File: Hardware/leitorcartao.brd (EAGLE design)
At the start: 34.5 x 68 mm, 168 parts, among them IC1 TL084, IC2 TL084, Q1 BSH103, Q2 BC847ASMD, Q3 BC857ALT1SMD, Q4 BC847ALT1SMD, Q5 BC847ALT1SMD, Q6 BC847ALT1SMD, Q7 BC847ALT1SMD, Q8 BC847ALT1SMD, U1 SAMD20E14A-AUT, U3 TLV1117-50CDCYR, U4 MFRC52202HN1, U5 LP2985-33DBVR, X1 ANTENA 125kHz, X2 MIFARE ANTENA

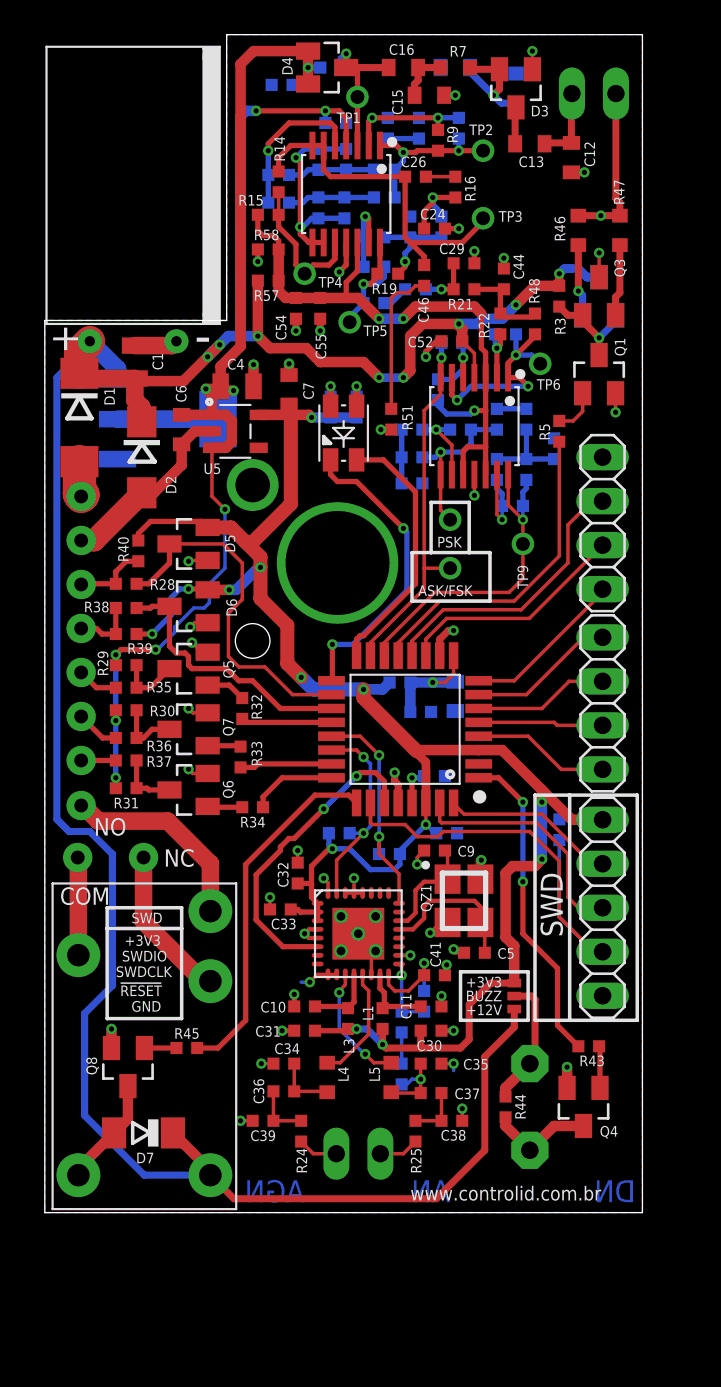
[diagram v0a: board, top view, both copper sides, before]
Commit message: Nova versão do leitor. Aguardando revisão.
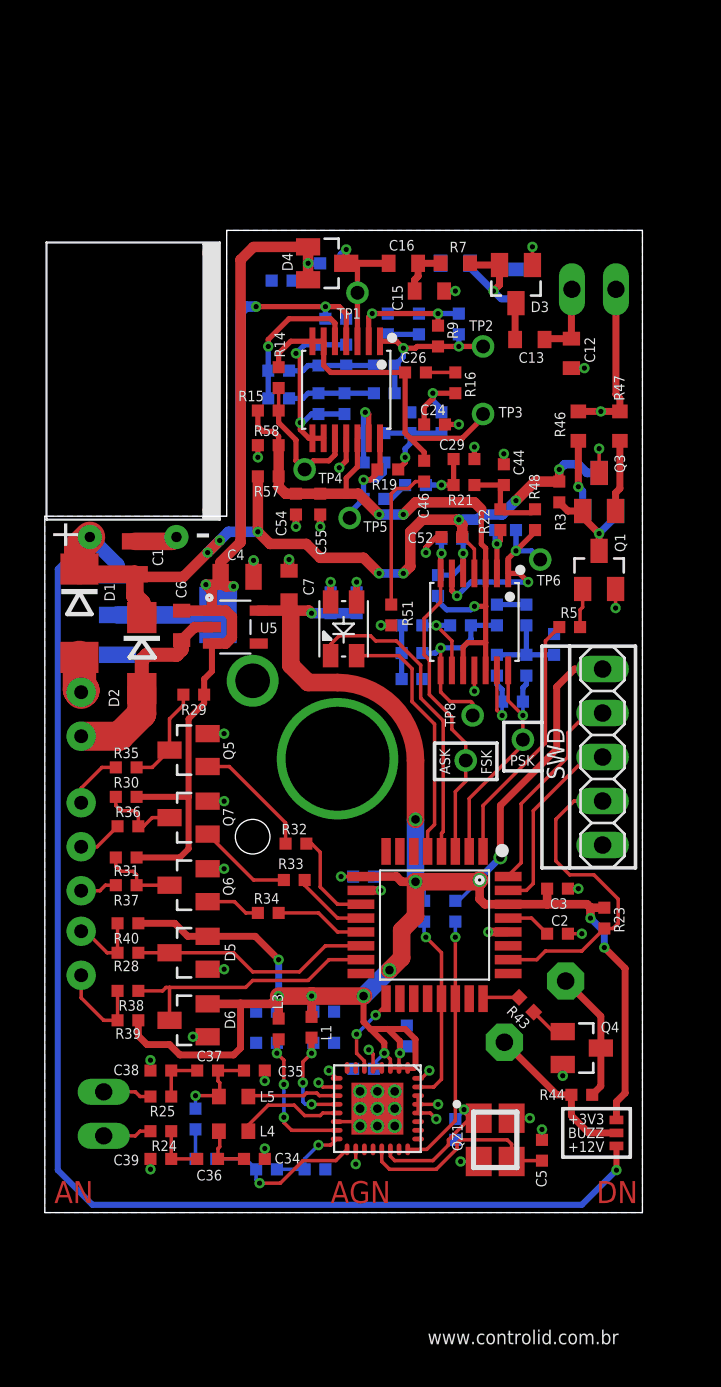
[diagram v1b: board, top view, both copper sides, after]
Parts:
- removed C43: 4.7uF, RFiD:C0603
- removed COM: COM, RFiD:HOLE
- removed D7: LL4148, RFiD:SOD80C
- removed L6: BEAD, RFiD:R0402
- removed NC: NC, RFiD:HOLE
- removed NO: NO, RFiD:HOLE
- removed Q8: BC847ALT1SMD, RFiD:SOT23
- removed R45: 2.2k, RFiD:R0402
- removed RL1: RELE, RFiD:RELE
- removed TOUCH-C, TOUCH-L: (no value), pinhead:1X04
- removed TP9: TESTPOINT, RFiD:TESTPOINT
- added TP8: TESTPOINT, RFiD:TESTPOINT
- moved D6 23.9 mm to (8.30, 11.1)
- moved D5 23.6 mm to (8.30, 15.0)
- moved R39 22.3 mm to (4.80, 11.1)
- moved R38 22.1 mm to (4.80, 12.8)
- moved R40 21.5 mm to (4.80, 16.7), turned to 180 degrees
- moved R28 21.3 mm to (4.80, 15.0)
- moved LED-IN 20.0 mm to (2.10, 16.2)
- moved MODE-SEL 20.0 mm to (2.10, 13.7)
- moved C38 17.0 mm to (6.70, 8.20), turned to 0 degrees
- moved C9 16.1 mm to (23.7, 4.80), flipped to the bottom, turned to 270 degrees
- moved X2 14.9 mm to (3.40, 5.70), turned to 270 degrees
- moved R25 14.8 mm to (6.70, 6.70), turned to 180 degrees
- moved QZ1 13.9 mm to (26.0, 4.20)
- moved C40 13.8 mm to (9.30, 3.10), turned to 180 degrees
- moved PSK 13.4 mm to (27.6, 27.3)
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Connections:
- removed net N$40: C42.1, C43.1, L6.1, U1.9
- removed net N$48: D7.A, Q8.3, RL1.1
- removed net N$49: Q8.1, R45.1
- removed net N$56: NO.P$1, RL1.3
- removed net N$57: NC.P$1, RL1.4
- removed net N$58: COM.P$1, RL1.2
- removed net RELE: R45.2, U1.25
- removed net TOUCH-C1: TOUCH-C.1, U1.8
- removed net TOUCH-C2: TOUCH-C.2, U1.11
- removed net TOUCH-C3: TOUCH-C.3, U1.12
- removed net TOUCH-L1: TOUCH-L.1, U1.4
- removed net TOUCH-L2: TOUCH-L.2, U1.5
- removed net TOUCH-L3: TOUCH-L.3, U1.6
- removed net TOUCH-L4: TOUCH-L.4, U1.7
- net +12V: no longer D7.C, RL1.5
- net +3V3: now also C42.1, U1.9; no longer L6.2, U1.3
- net 125KHZ-ANTENA: now also U1.1; no longer U1.13
- net ASK-FSK: now also U1.3; no longer U1.15
- net BUZZER: now also U1.24; no longer U1.1
- net CARD-PRES: now also U1.13; no longer U1.24
- net D0/TX/CLK: now also U1.11; no longer U1.20
- net D1/DATA: now also U1.12; no longer U1.23
- net GND: no longer C43.2, Q8.2, TOUCH-C.4
- net LED-GREEN-CTRL: now also U1.5; no longer U1.16
- net LED-INPUT: now also U1.14; no longer U1.18
- net LED-RED-CTRL: now also U1.4; no longer U1.17
- net MIFARE-RST: now also U1.17; no longer U1.27
- net MIFARE-SCL: now also U1.21; no longer U1.22
- net MIFARE-SDA: now also U1.22; no longer U1.21
- net N$2: now also U4.12; no longer U4.15
- net N$38: now also X2.2; no longer X2.1
- net N$39: now also X2.1; no longer X2.2
- net N$4: now also U4.15; no longer U4.12
- net N$71: now also TP8.P$1; no longer PSK.P$1
- net PSK: now also PSK.P$1, U1.2; no longer TP9.P$1, U1.14
- net USART-RX: now also U1.15; no longer U1.19
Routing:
- net RELE: track 20.7 -> 0.00 mm
- net +3V3: track 117.2 -> 134.3 mm, vias 13 -> 15
- net TOUCH-C3: track 16.5 -> 0.00 mm
- net BUZZER: track 18.6 -> 2.11 mm, vias 2 -> 0
- net +12V: track 160.3 -> 146.3 mm, vias 10 -> 11
- net TOUCH-C2: track 13.4 -> 0.00 mm
- net MIFARE-RST: track 18.2 -> 4.89 mm
- net N$56: track 11.6 -> 0.00 mm
- net TOUCH-C1: track 9.45 -> 0.00 mm
- net GND: track 63.2 -> 54.1 mm, vias 52 -> 51
- net N$57: track 8.98 -> 0.00 mm
- net RESET: track 27.5 -> 18.7 mm
- net TOUCH-L4: track 8.52 -> 0.00 mm
- net TOUCH-L1: track 7.94 -> 0.00 mm
- net TOUCH-L3: track 7.80 -> 0.00 mm
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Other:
- board size 34.5 x 68 mm -> 34.5 x 56.7 mm
- board text added: "ASK"
- board text added: "FSK"
